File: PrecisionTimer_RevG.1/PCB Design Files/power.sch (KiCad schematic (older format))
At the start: 52 parts, among them Q1 NMOS 2A, U10 MIC2095-2YMT-TR, U4 ATSAM4S2, U5 TS30012-M050QFNR, U6 MIC23050-SYML-TR, U7 MIC23050-4YML-TR, U8 LM74610QDGKTQ1, U9 MIC2095-2YMT-TR

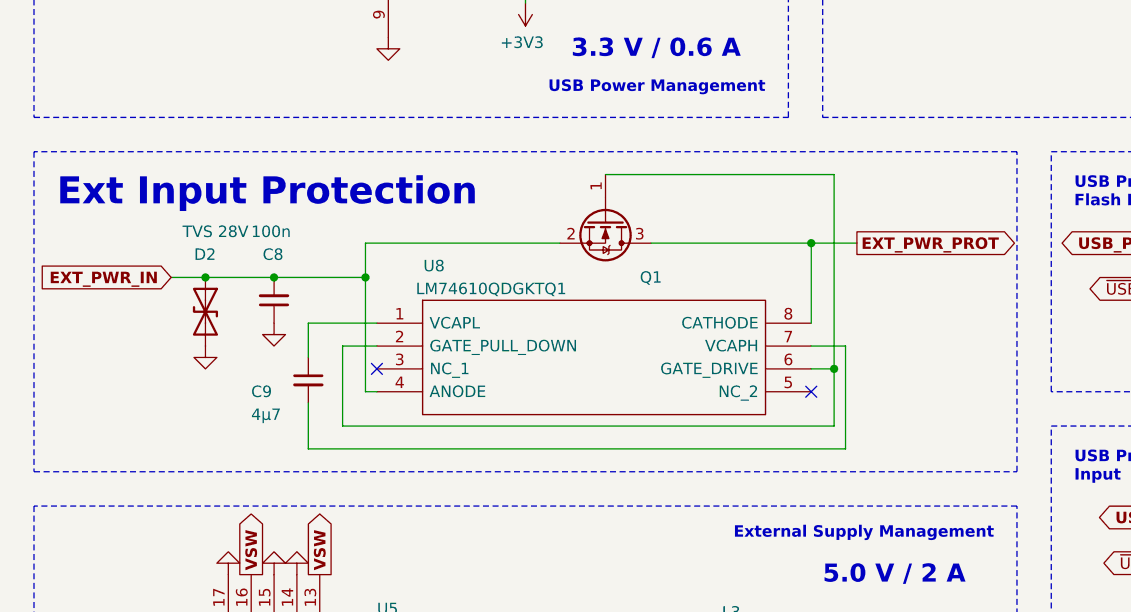
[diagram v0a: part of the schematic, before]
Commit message: Add files via upload
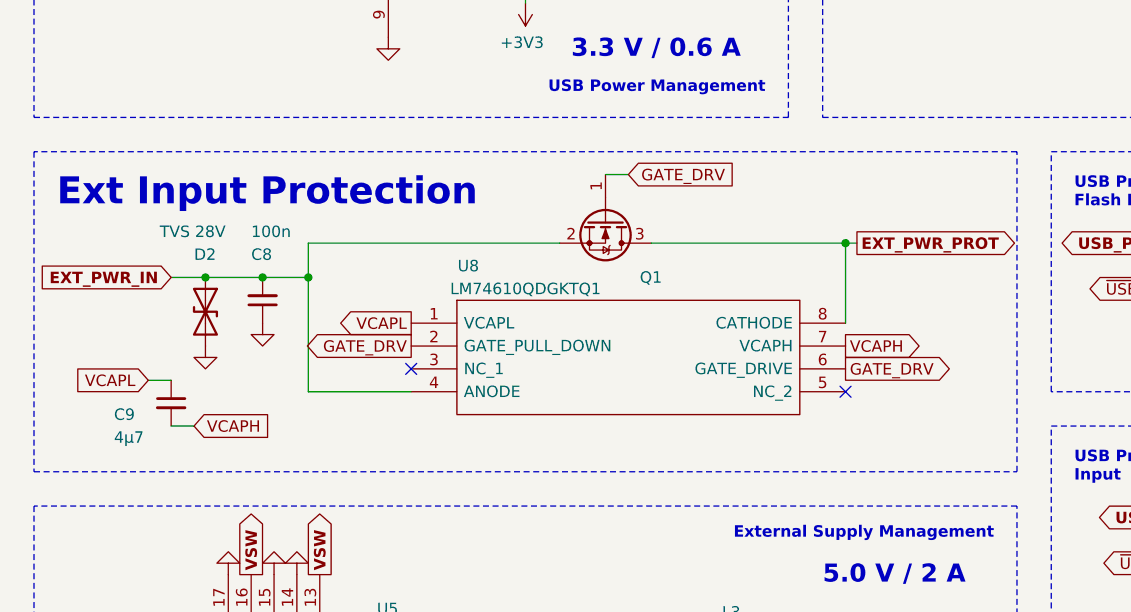
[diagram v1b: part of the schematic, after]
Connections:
- net VCAPL: now reaches C9.1, U8.1 (VCAPL)
- net GATE_DRV: now reaches Q1.1 (G), U8.2 (GATE_PULL_DOWN), U8.6 (GATE_DRIVE)
- net VCAPH: now reaches C9.2, U8.7 (VCAPH)
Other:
- moved on the sheet: C8, C9, U8
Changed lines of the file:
@@
 L SamacSys_Parts:LM74610QDGKTQ1 U?
 U 1 1 5FAA3A27
-P 2550 3350
+P 2700 3350
 AR Path="/5FAA3A27" Ref="U?"  Part="1"
 AR Path="/5F82CBFD/5FAA3A27" Ref="U8"  Part="1"
-F 0 "U8" H 2800 3600 50  0000 C CNN
-F 1 "LM74610QDGKTQ1" H 3050 3500 50  0000 C CNN
-F 2 "SamacSys_Parts:SOP65P490X110-8N" H 4300 3450 50  0001 L CNN
-F 3 "http://www.ti.com/lit/ds/symlink/lm74610-q1.pdf" H 4300 3350 50  0001 L CNN
-F 4 "TEXAS INSTRUMENTS - LM74610QDGKTQ1 - DIODE-OR CNTRL, 100V, VSSOP-8" H 4300 3250 50  0001 L CNN "Description"
-F 5 "1.1" H 4300 3150 50  0001 L CNN "Height"
-F 6 "Texas Instruments" H 4300 3050 50  0001 L CNN "Manufacturer_Name"
-F 7 "LM74610QDGKTQ1" H 4300 2950 50  0001 L CNN "Manufacturer_Part_Number"
-F 8 "595-LM74610QDGKTQ1" H 4300 2850 50  0001 L CNN "Mouser Part Number"
-F 9 "https://www.mouser.co.uk/ProductDetail/Texas-Instruments/LM74610QDGKTQ1?qs=3jdCaFhktORzOMycfF4DBg%3D%3D" H 4300 2750 50  0001 L CNN "Mouser Price/Stock"
-F 10 "1330675P" H 4300 2650 50  0001 L CNN "RS Part Number"
-F 11 "http://uk.rs-online.com/web/p/products/1330675P" H 4300 2550 50  0001 L CNN "RS Price/Stock"
-	1    2550 3350
+F 0 "U8" H 2950 3600 50  0000 C CNN
+F 1 "LM74610QDGKTQ1" H 3200 3500 50  0000 C CNN
+F 2 "SamacSys_Parts:SOP65P490X110-8N" H 4450 3450 50  0001 L CNN
+F 3 "http://www.ti.com/lit/ds/symlink/lm74610-q1.pdf" H 4450 3350 50  0001 L CNN
+F 4 "TEXAS INSTRUMENTS - LM74610QDGKTQ1 - DIODE-OR CNTRL, 100V, VSSOP-8" H 4450 3250 50  0001 L CNN "Description"
+F 5 "1.1" H 4450 3150 50  0001 L CNN "Height"
+F 6 "Texas Instruments" H 4450 3050 50  0001 L CNN "Manufacturer_Name"
+F 7 "LM74610QDGKTQ1" H 4450 2950 50  0001 L CNN "Manufacturer_Part_Number"
+F 8 "595-LM74610QDGKTQ1" H 4450 2850 50  0001 L CNN "Mouser Part Number"
+F 9 "https://www.mouser.co.uk/ProductDetail/Texas-Instruments/LM74610QDGKTQ1?qs=3jdCaFhktORzOMycfF4DBg%3D%3D" H 4450 2750 50  0001 L CNN "Mouser Price/Stock"
+F 10 "1330675P" H 4450 2650 50  0001 L CNN "RS Part Number"
+F 11 "http://uk.rs-online.com/web/p/products/1330675P" H 4450 2550 50  0001 L CNN "RS Price/Stock"
+	1    2700 3350
 	1    0    0    -1
 $EndComp
@@
 AR Path="/5F82CBFD/5FAA3A2D" Ref="D2"  Part="1"
 F 0 "D2" V 1550 3250 50  0000 L CNN
-F 1 "TVS 28V" V 1450 3200 50  0000 L CNN
+F 1 "TVS 28V" V 1450 3100 50  0000 L CNN
 F 2 "Diode_SMD:D_SMB" H 1800 3300 50  0001 C CNN
 F 3 "~" H 1800 3300 50  0001 C CNN
@@
 L Device:C_Small C?
 U 1 1 5FAA3A33
-P 2250 3600
+P 1650 3700
 AR Path="/5FAA3A33" Ref="C?"  Part="1"
 AR Path="/5F82CBFD/5FAA3A33" Ref="C9"  Part="1"
-F 0 "C9" H 2000 3550 50  0000 L CNN
-F 1 "4µ7" H 2000 3450 50  0000 L CNN
-F 2 "Capacitor_SMD:C_0603_1608Metric" H 2250 3600 50  0001 C CNN
-F 3 "~" H 2250 3600 50  0001 C CNN
-	1    2250 3600
-	1    0    0    -1
-$EndComp
-Wire Wire Line
-	2550 3350 2250 3350
-Wire Wire Line
-	2250 3350 2250 3500
-Wire Wire Line
-	2250 3700 2250 3900
-Wire Wire Line
-	2250 3900 4600 3900
-Wire Wire Line
-	4600 3900 4600 3450
-Wire Wire Line
-	4600 3450 4450 3450
-Wire Wire Line
-	2550 3450 2400 3450
-Wire Wire Line
-	2400 3450 2400 3800
-Wire Wire Line
-	2400 3800 4550 3800
-Wire Wire Line
-	4550 3800 4550 3550
-Wire Wire Line
-	4550 3550 4450 3550
-Wire Wire Line
-	4550 2700 3550 2700
-Wire Wire Line
-	4450 3350 4450 3000
-Wire Wire Line
-	4450 3000 3750 3000
-Wire Wire Line
-	3350 3000 2500 3000
-Wire Wire Line
-	2500 3000 2500 3150
-Wire Wire Line
-	2500 3150 2500 3650
-Wire Wire Line
-	2500 3650 2550 3650
+F 0 "C9" H 1400 3650 50  0000 L CNN
+F 1 "4µ7" H 1400 3550 50  0000 L CNN
+F 2 "Capacitor_SMD:C_0603_1608Metric" H 1650 3700 50  0001 C CNN
+F 3 "~" H 1650 3700 50  0001 C CNN
+	1    1650 3700
+	1    0    0    -1
+$EndComp
+Wire Wire Line
+	3650 2700 3550 2700
+Wire Wire Line
+	4600 3350 4600 3000
+Wire Wire Line
+	3350 3000 2250 3000
+Wire Wire Line
+	2250 3000 2250 3150
 $Comp
 L Device:C_Small C?
 U 1 1 5FAA3A4B
-P 2100 3250
+P 2050 3250
 AR Path="/5FAA3A4B" Ref="C?"  Part="1"
 AR Path="/5F82CBFD/5FAA3A4B" Ref="C8"  Part="1"
-F 0 "C8" H 2150 3050 50  0000 R CNN
-F 1 "100n" H 2200 2950 50  0000 R CNN
-F 2 "Capacitor_SMD:C_0603_1608Metric" H 2100 3250 50  0001 C CNN
-F 3 "~" H 2100 3250 50  0001 C CNN
-	1    2100 3250
+F 0 "C8" H 2100 3050 50  0000 R CNN
+F 1 "100n" H 2100 2950 50  0000 R CNN
+F 2 "Capacitor_SMD:C_0603_1608Metric" H 2050 3250 50  0001 C CNN
+F 3 "~" H 2050 3250 50  0001 C CNN
+	1    2050 3250
 	-1   0    0    1
 $EndComp
@@
 Wire Wire Line
 	1650 3150 1800 3150
-Connection ~ 2500 3150
 Connection ~ 1800 3150
 Wire Wire Line
-	1800 3150 2100 3150
-Connection ~ 2100 3150
-Wire Wire Line
-	2100 3150 2500 3150
+	1800 3150 2050 3150
 $Comp
 L power:GND #PWR?
@@
 L power:GND #PWR?
 U 1 1 5FAA3A5E
-P 2100 3350
+P 2050 3350
 AR Path="/5FAA3A5E" Ref="#PWR?"  Part="1"
 AR Path="/5F82CBFD/5FAA3A5E" Ref="#PWR059"  Part="1"
-F 0 "#PWR059" H 2100 3100 50  0001 C CNN
-F 1 "GND" H 2105 3177 50  0001 C CNN
-F 2 "" H 2100 3350 50  0001 C CNN
-F 3 "" H 2100 3350 50  0001 C CNN
-	1    2100 3350
+F 0 "#PWR059" H 2050 3100 50  0001 C CNN
+F 1 "GND" H 2055 3177 50  0001 C CNN
+F 2 "" H 2050 3350 50  0001 C CNN
+F 3 "" H 2050 3350 50  0001 C CNN
+	1    2050 3350
 	-1   0    0    -1
 $EndComp
 Text GLabel 4650 3000 2    50   Output ~ 10
 EXT_PWR_PROT
-Wire Wire Line
-	4450 3000 4650 3000
-Connection ~ 4450 3000
-Wire Wire Line
-	4550 2700 4550 3550
-Connection ~ 4550 3550
-NoConn ~ 2550 3550
-NoConn ~ 4450 3650
+NoConn ~ 2700 3550
+NoConn ~ 4600 3650
 $Comp
 L Device:Q_NMOS_GSD Q?
@@
 	7450 6250 7550 6250
 Connection ~ 7550 6250
+Text GLabel 4600 3550 2    50   Output ~ 0
+GATE_DRV
+Text GLabel 4600 3450 2    50   Output ~ 0
+VCAPH
+Text GLabel 2700 3350 0    50   Output ~ 0
+VCAPL
+Text GLabel 1550 3600 0    50   Input ~ 0
+VCAPL
+Text GLabel 2700 3450 0    50   Output ~ 0
+GATE_DRV
+Text GLabel 3650 2700 2    50   Input ~ 0
+GATE_DRV
+Connection ~ 2050 3150
+Wire Wire Line
+	2050 3150 2250 3150
+Connection ~ 4600 3000
+Wire Wire Line
+	4600 3000 4650 3000
+Wire Wire Line
+	3750 3000 4600 3000
+Wire Wire Line
+	2250 3650 2700 3650
+Wire Wire Line
+	2250 3150 2250 3650
+Connection ~ 2250 3150
+Wire Wire Line
+	1550 3600 1650 3600
+Wire Wire Line
+	1650 3800 1750 3800
+Text GLabel 1750 3800 2    50   Input ~ 0
+VCAPH
 $EndSCHEMATC
